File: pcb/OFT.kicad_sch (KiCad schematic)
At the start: 28 parts, among them J1 Conn_01x04_Pin, J2 IF-D92, J3 IF-E91A, U1 SN74LVC1G14, U4 SN74LVC1G14, U5 NE555D, U6 NE555D

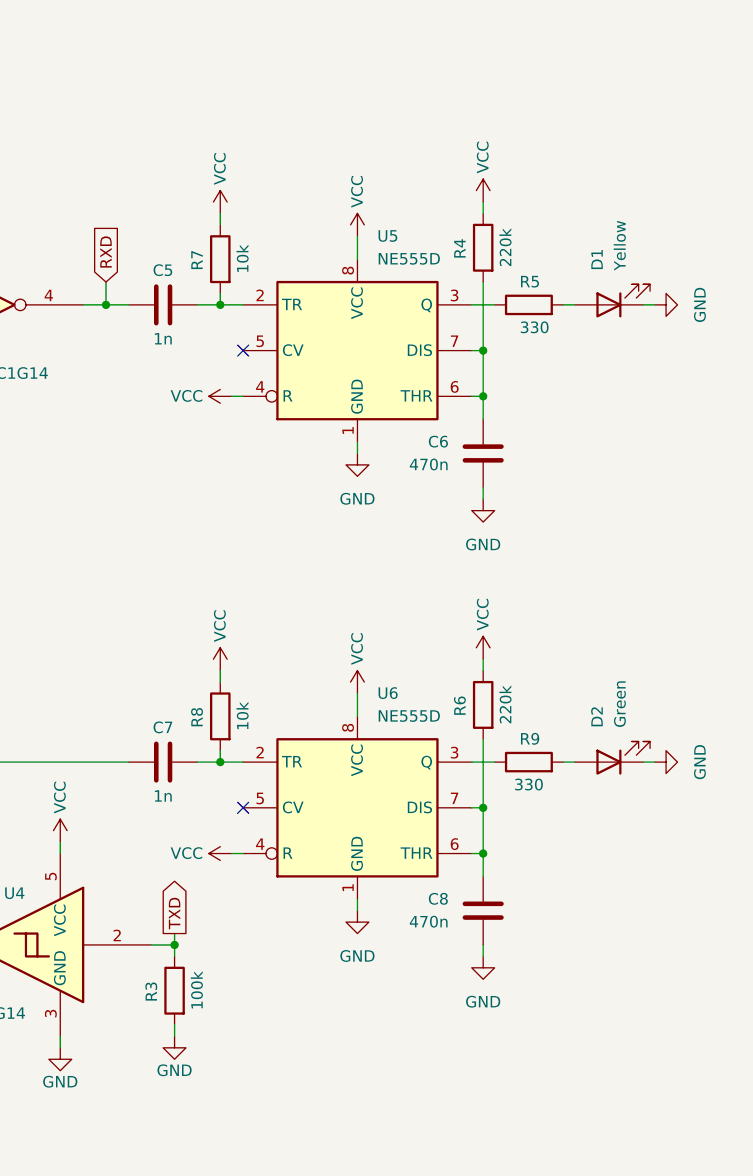
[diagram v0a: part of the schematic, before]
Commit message: Update to KiCAD 9
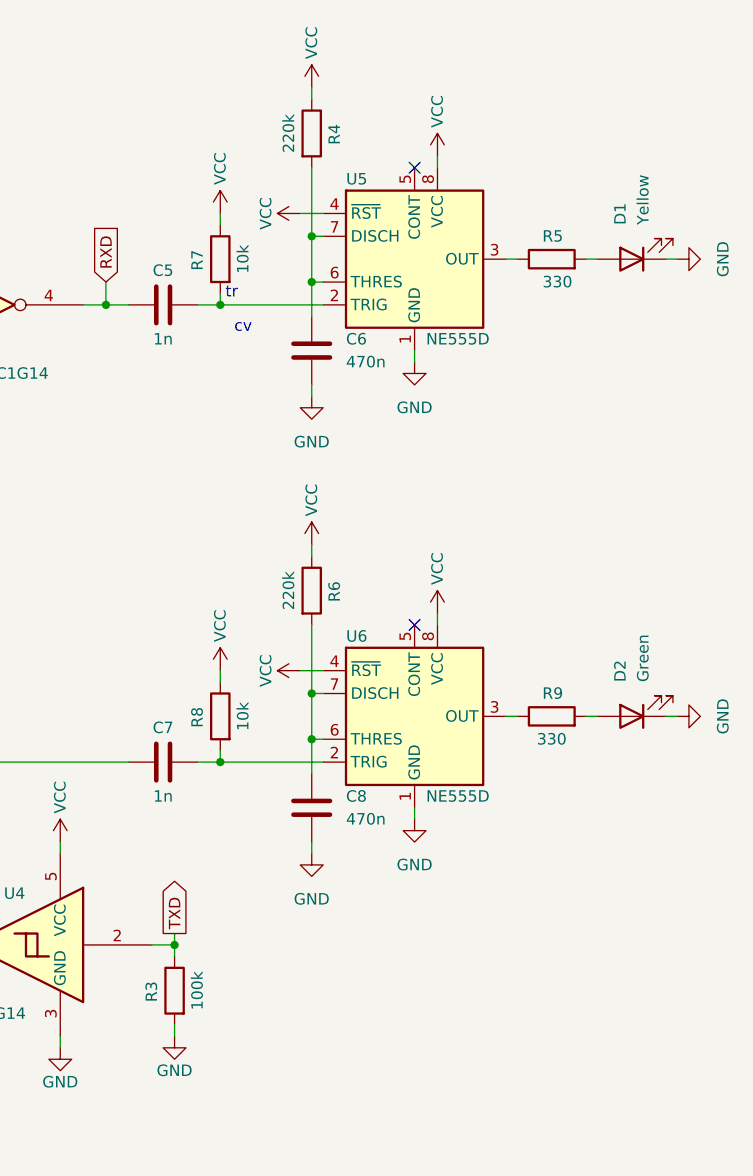
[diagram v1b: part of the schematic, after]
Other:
- note added: "cv"
- note added: "tr"
- moved on the sheet: C6, C8, D1, D2, R4, R5, R6, R9

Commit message: Rename/Add/Remove bom fields
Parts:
- C1, C2, C3, C4: HTL (none) -> 100128; Vendor HTL -> (none); VendorId 100128 -> (none)
- C5, C7: HTL (none) -> 102542; Vendor HTL -> (none); VendorId 102542 -> (none)
- C6, C8: HTL (none) -> 103260; Vendor HTL -> (none); VendorId 103260 -> (none)
- D1, D2: HTL (none) -> 100438, 100440; Vendor HTL -> (none); VendorId 100438, 100440 -> (none)
- D3: HTL (none) -> 100194; Vendor HTL -> (none); VendorId 100194 -> (none)
- FID4: now left out of the parts list
- J1: HTL (none) -> 101523; Vendor HTL -> (none); VendorId 101523 -> (none)
- J2, J3: HTL (none) -> 103594; Vendor HTL -> (none); VendorId 103594 -> (none)
- R1: HTL (none) -> 102956; Vendor HTL -> (none); VendorId 102956 -> (none)
- R2: HTL (none) -> 102937; Vendor HTL -> (none); VendorId 102937 -> (none)
- R3: HTL (none) -> 102987; Vendor HTL -> (none); VendorId 102987 -> (none)
- R4, R6: HTL (none) -> 102991; Vendor HTL -> (none); VendorId 102991 -> (none)
- R5, R9: HTL (none) -> 102940; Vendor HTL -> (none); VendorId 102940 -> (none)
- R7, R8: HTL (none) -> 102967; Vendor HTL -> (none); VendorId 102967 -> (none)
- U1, U4: HTL (none) -> 103595; Vendor HTL -> (none); VendorId 103595 -> (none)
- U5, U6: HTL (none) -> 100328; Vendor HTL -> (none); VendorId 100328 -> (none)
